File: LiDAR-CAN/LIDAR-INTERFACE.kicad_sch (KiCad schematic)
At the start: 31 parts, among them U3 W5500, Y1 25MHz

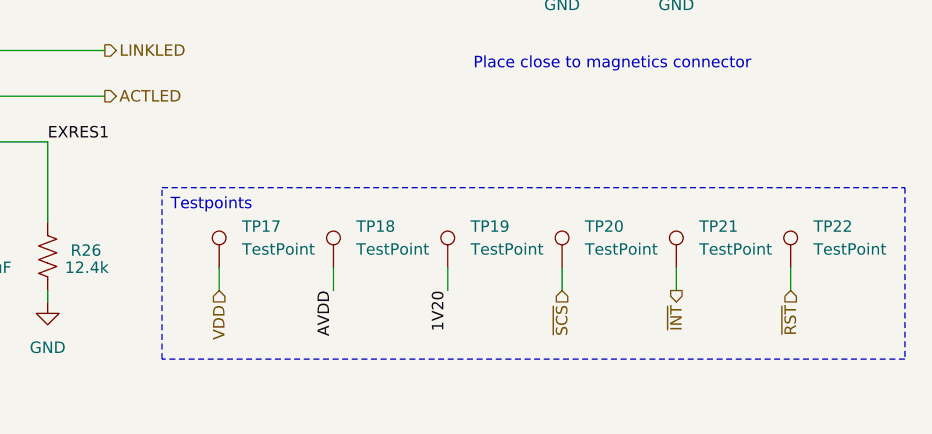
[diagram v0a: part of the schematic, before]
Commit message: Update complete first placement
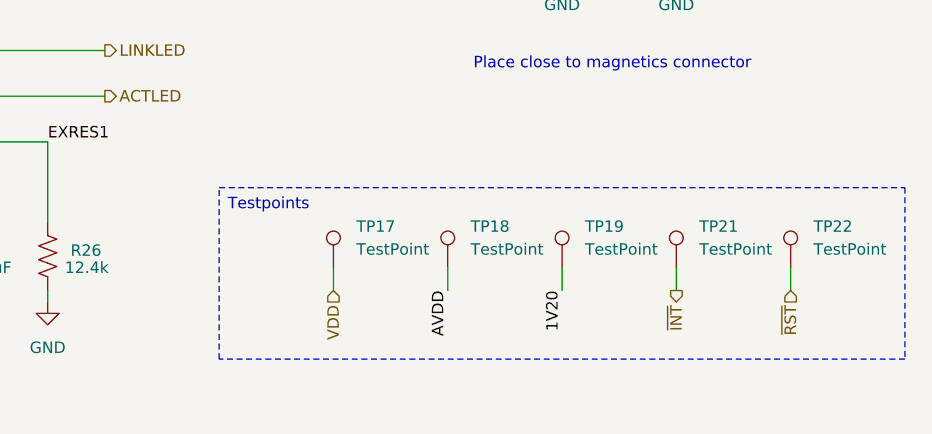
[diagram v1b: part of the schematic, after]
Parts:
- removed TP20: TestPoint, TestPoint:TestPoint_Pad_D1.0mm, symbol Connector:TestPoint
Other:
- moved on the sheet: TP17, TP18, TP19
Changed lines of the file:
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@@
 	(text_box "Testpoints"
 		(exclude_from_sim no)
-		(at 196.85 139.7 0)
-		(size 82.55 19.05)
+		(at 203.2 139.7 0)
+		(size 76.2 19.05)
 		(margins 0.9525 0.9525 0.9525 0.9525)
 		(stroke
@@
 	(wire
 		(pts
-			(xy 215.9 148.59) (xy 215.9 151.13)
+			(xy 228.6 148.59) (xy 228.6 151.13)
 		)
 		(stroke
@@
 	(wire
 		(pts
-			(xy 241.3 148.59) (xy 241.3 151.13)
-		)
-		(stroke
-			(width 0)
-			(type default)
-		)
-	)
-	(wire
-		(pts
 			(xy 76.2 50.8) (xy 76.2 53.34)
 		)
@@
 	(wire
 		(pts
-			(xy 228.6 148.59) (xy 228.6 151.13)
+			(xy 241.3 148.59) (xy 241.3 151.13)
 		)
 		(stroke
@@
 	(wire
 		(pts
-			(xy 203.2 148.59) (xy 203.2 151.13)
+			(xy 215.9 148.59) (xy 215.9 151.13)
 		)
 		(stroke
@@
 	)
 	(label "1V20"
-		(at 228.6 151.13 270)
+		(at 241.3 151.13 270)
 		(effects
 			(font
@@
 	)
 	(label "AVDD"
-		(at 215.9 151.13 270)
+		(at 228.6 151.13 270)
 		(effects
 			(font
@@
 	(hierarchical_label "~{SCS}"
 		(shape input)
-		(at 241.3 151.13 270)
-		(effects
-			(font
-				(size 1.27 1.27)
-			)
-			(justify right)
-		)
-	)
-	(hierarchical_label "~{SCS}"
-		(shape input)
 		(at 114.3 91.44 180)
 		(effects
@@
 	(hierarchical_label "VDD"
 		(shape input)
-		(at 203.2 151.13 270)
+		(at 215.9 151.13 270)
 		(effects
 			(font
@@
 	)
 	(symbol
-		(lib_id "Connector:TestPoint")
-		(at 241.3 148.59 0)
-		(unit 1)
-		(exclude_from_sim no)
-		(in_bom no)
-		(on_board yes)
-		(dnp no)
-		(fields_autoplaced yes)
-		(property "Reference" "TP20"
-			(at 243.84 144.0179 0)
-			(effects
-				(font
-					(size 1.27 1.27)
-				)
-				(justify left)
-			)
-		)
-		(property "Value" "TestPoint"
-			(at 243.84 146.5579 0)
-			(effects
-				(font
-					(size 1.27 1.27)
-				)
-				(justify left)
-			)
-		)
-		(property "Footprint" "TestPoint:TestPoint_Pad_D1.0mm"
-			(at 246.38 148.59 0)
-			(effects
-				(font
-					(size 1.27 1.27)
-				)
-				(hide yes)
-			)
-		)
-		(property "Datasheet" "~"
-			(at 246.38 148.59 0)
-			(effects
-				(font
-					(size 1.27 1.27)
-				)
-				(hide yes)
-			)
-		)
-		(property "Description" "test point"
-			(at 241.3 148.59 0)
-			(effects
-				(font
-					(size 1.27 1.27)
-				)
-				(hide yes)
-			)
-		)
-		(pin "1"
-		)
-		(instances
-			(project "LiDAR-CAN"
-				(path "/56db6f21-0e4a-4321-bd8a-db37f1842dd9/91fe436f-7e8c-47e0-899c-e39330e04729"
-					(reference "TP20")
-					(unit 1)
-				)
-			)
-		)
-	)
-	(symbol
 		(lib_id "Symbols:CAP CER 0.1UF 50V X7R 0603")
 		(at 127 57.15 180)
@@
 	(symbol
 		(lib_id "Connector:TestPoint")
-		(at 228.6 148.59 0)
+		(at 241.3 148.59 0)
 		(unit 1)
 		(exclude_from_sim no)
@@
 		(fields_autoplaced yes)
 		(property "Reference" "TP19"
-			(at 231.14 144.0179 0)
+			(at 243.84 144.0179 0)
 			(effects
 				(font
@@
 		)
 		(property "Value" "TestPoint"
-			(at 231.14 146.5579 0)
+			(at 243.84 146.5579 0)
 			(effects
 				(font
@@
 		)
 		(property "Footprint" "TestPoint:TestPoint_Pad_D1.0mm"
-			(at 233.68 148.59 0)
+			(at 246.38 148.59 0)
 			(effects
 				(font
@@
 		)
 		(property "Datasheet" "~"
-			(at 233.68 148.59 0)
+			(at 246.38 148.59 0)
 			(effects
 				(font
@@
 		)
 		(property "Description" "test point"
-			(at 228.6 148.59 0)
+			(at 241.3 148.59 0)
 			(effects
 				(font
@@
 	(symbol
 		(lib_id "Connector:TestPoint")
-		(at 203.2 148.59 0)
+		(at 215.9 148.59 0)
 		(unit 1)
 		(exclude_from_sim no)
@@
 		(fields_autoplaced yes)
 		(property "Reference" "TP17"
-			(at 205.74 144.0179 0)
+			(at 218.44 144.0179 0)
 			(effects
 				(font
@@
 		)
 		(property "Value" "TestPoint"
-			(at 205.74 146.5579 0)
+			(at 218.44 146.5579 0)
 			(effects
 				(font
@@
 		)
 		(property "Footprint" "TestPoint:TestPoint_Pad_D1.0mm"
-			(at 208.28 148.59 0)
+			(at 220.98 148.59 0)
 			(effects
 				(font
@@
 		)
 		(property "Datasheet" "~"
-			(at 208.28 148.59 0)
+			(at 220.98 148.59 0)
 			(effects
 				(font
@@
 		)
 		(property "Description" "test point"
-			(at 203.2 148.59 0)
+			(at 215.9 148.59 0)
 			(effects
 				(font
@@
 	(symbol
 		(lib_id "Connector:TestPoint")
-		(at 215.9 148.59 0)
+		(at 228.6 148.59 0)
 		(unit 1)
 		(exclude_from_sim no)
@@
 		(fields_autoplaced yes)
 		(property "Reference" "TP18"
-			(at 218.44 144.0179 0)
+			(at 231.14 144.0179 0)
 			(effects
 				(font
@@
 		)
 		(property "Value" "TestPoint"
-			(at 218.44 146.5579 0)
+			(at 231.14 146.5579 0)
 			(effects
 				(font
@@
 		)
 		(property "Footprint" "TestPoint:TestPoint_Pad_D1.0mm"
-			(at 220.98 148.59 0)
+			(at 233.68 148.59 0)
 			(effects
 				(font
@@
 		)
 		(property "Datasheet" "~"
-			(at 220.98 148.59 0)
+			(at 233.68 148.59 0)
 			(effects
 				(font
@@
 		)
 		(property "Description" "test point"
-			(at 215.9 148.59 0)
+			(at 228.6 148.59 0)
 			(effects
 				(font
